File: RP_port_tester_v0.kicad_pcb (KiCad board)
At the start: 2 copper layers, 82 parts, among them J1 USB_B PORT0, J2 USB_B PORT1, J3 USB_B PORT2, J4 USB_B PORT3, J5 DE9_Pins, J6 DE9_Pins, J7 DE9_Pins, J8 DE9_Pins, J9 UART, Q1 IRLZ44N, SW1 BOOTSEL, U1 AMS1117-3.3, U2 STMPS2151, U3 STMPS2151, U4 FSUSB74MPX, U5 W25Q128JVS, U6 STMPS2151, U7 RP2040, U8 LM2904, Y1 ABM8-272-T3

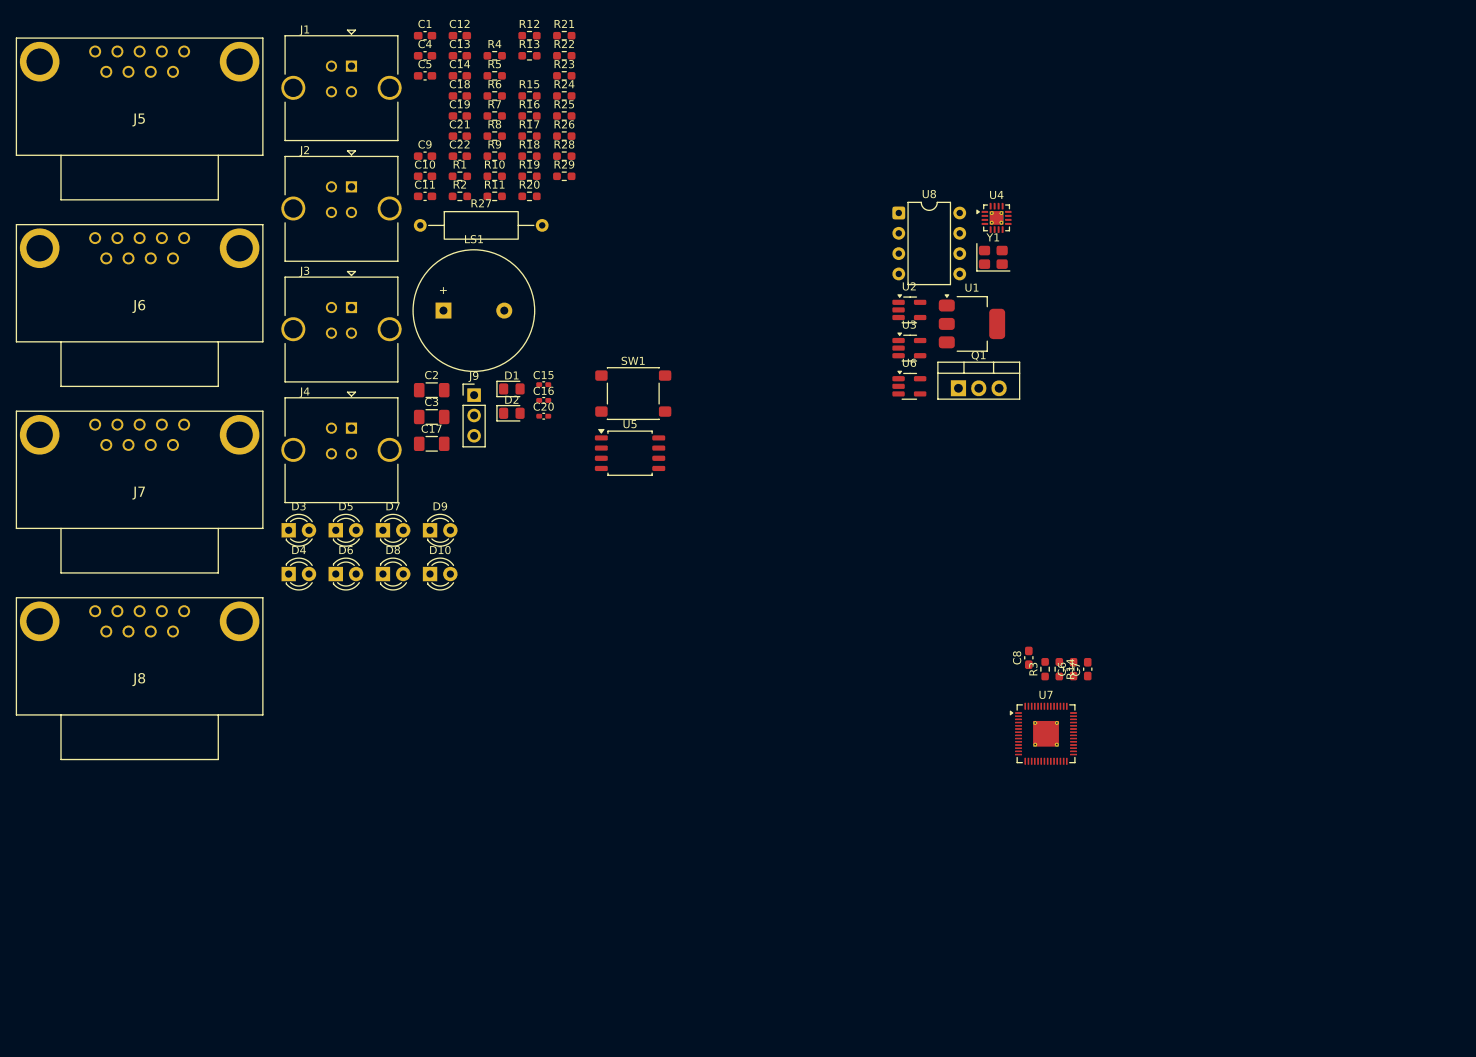
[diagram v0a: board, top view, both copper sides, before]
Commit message: Layout and Tracing
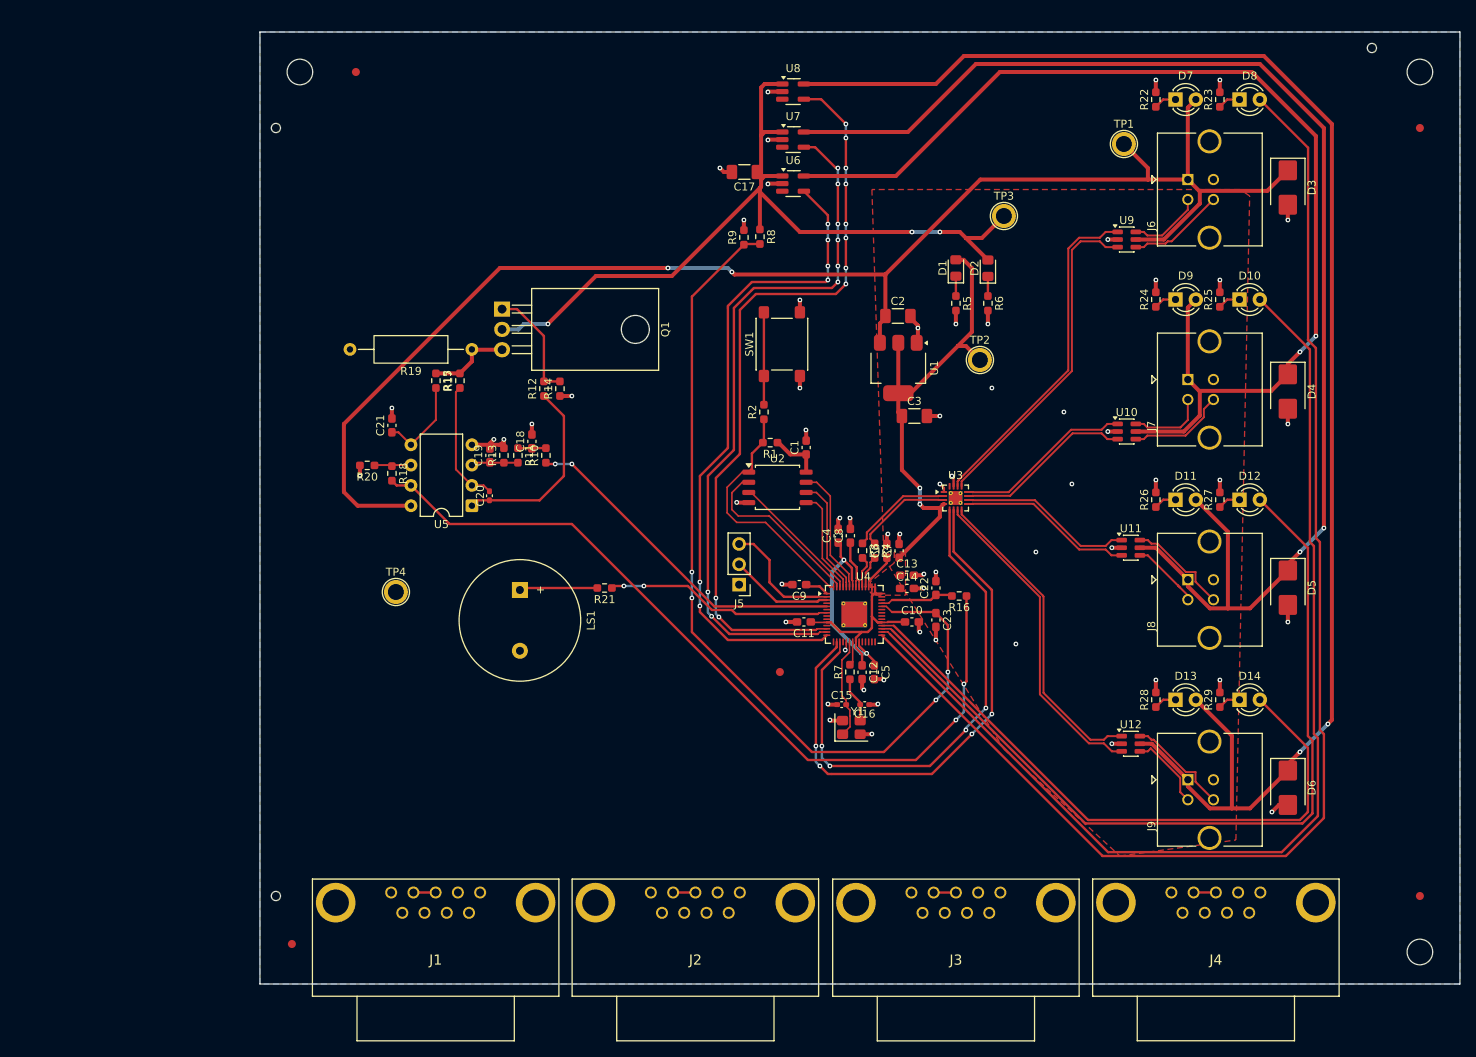
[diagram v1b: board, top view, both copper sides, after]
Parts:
- removed the J1 at (81.4, 29.3)
- removed the J2 at (81.4, 44.4)
- removed the J3 at (81.4, 59.4)
- removed the J4 at (81.4, 74.5)
- removed the R6 at (99.3, 33.0)
- removed the R7 at (99.3, 35.5)
- removed the U2 at (151.2, 59.7)
- removed the U3 at (151.2, 64.5)
- added C23: 100n, Capacitor_SMD:C_0603_1608Metric_Pad1.08x0.95mm_HandSolder, F.Cu at (154.5, 98.5)
- added D3: P6SMB6.8, Diode_SMD:D_SMB, F.Cu at (198.5, 44.4)
- added D4: P6SMB6.8, Diode_SMD:D_SMB, F.Cu at (198.5, 69.9)
- added D5: P6SMB6.8, Diode_SMD:D_SMB, F.Cu at (198.5, 94.5)
- added D6: P6SMB6.8, Diode_SMD:D_SMB, F.Cu at (198.5, 119.5)
- added FID1: Fiducial, Fiducial:Fiducial_1mm_Mask2mm, F.Cu at (74.0, 139.0)
- added FID2: Fiducial, Fiducial:Fiducial_1mm_Mask2mm, F.Cu at (82.0, 30.0)
- added FID3: Fiducial, Fiducial:Fiducial_1mm_Mask2mm, F.Cu at (215.0, 37.0)
- added FID4: Fiducial, Fiducial:Fiducial_1mm_Mask2mm, F.Cu at (215.0, 133.0)
- added FID5: Fiducial, Fiducial:Fiducial_1mm_Mask2mm, F.Cu at (135.0, 105.0)
- added H1: TOOLING_HOLE, MountingHole:ToolingHole_1.152mm, F.Cu at (209.0, 27.0)
- added H2: MountingHole, MountingHole:MountingHole_3.2mm_M3, F.Cu at (75.0, 30.0)
- added H3: TOOLING_HOLE, MountingHole:ToolingHole_1.152mm, F.Cu at (72.0, 37.0)
- added H4: MountingHole, MountingHole:MountingHole_3.2mm_M3, F.Cu at (215.0, 30.0)
- added H5: TOOLING_HOLE, MountingHole:ToolingHole_1.152mm, F.Cu at (72.0, 133.0)
- added H6: MountingHole, MountingHole:MountingHole_3.2mm_M3, F.Cu at (215.0, 140.0)
- added J6: USB_B PORT0, My_Library:USB_B_Vertical, F.Cu at (186.0, 43.4)
- added J7: USB_B PORT1, My_Library:USB_B_Vertical, F.Cu at (186.0, 68.4)
- added J8: USB_B PORT2, My_Library:USB_B_Vertical, F.Cu at (186.0, 93.5)
- added J9: USB_B PORT3, My_Library:USB_B_Vertical, F.Cu at (186.0, 118.5)
- added R14: 100k, Resistor_SMD:R_0603_1608Metric_Pad0.98x0.95mm_HandSolder, F.Cu at (107.5, 69.6)
- added R15: 1k, Resistor_SMD:R_0603_1608Metric_Pad0.98x0.95mm_HandSolder, F.Cu at (92.0, 68.6)
- added TP1: TestPoint, TestPoint:TestPoint_Plated_Hole_D2.0mm, F.Cu at (178.0, 39.0)
- added TP2: TestPoint, TestPoint:TestPoint_Plated_Hole_D2.0mm, F.Cu at (160.0, 66.0)
- added TP3: TestPoint, TestPoint:TestPoint_Plated_Hole_D2.0mm, F.Cu at (163.0, 48.0)
- added TP4: TestPoint, TestPoint:TestPoint_Plated_Hole_D2.0mm, F.Cu at (87.0, 95.0)
- added U10: USBLC6-2SC6, Package_TO_SOT_SMD:SOT-23-6, F.Cu at (178.4, 74.9)
- added U11: USBLC6-2SC6, Package_TO_SOT_SMD:SOT-23-6, F.Cu at (178.9, 89.5)
- added U12: USBLC6-2SC6, Package_TO_SOT_SMD:SOT-23-6, F.Cu at (178.9, 114.0)
- added U7: STMPS2151, Package_TO_SOT_SMD:SOT-23-5_HandSoldering, F.Cu at (136.7, 38.5)
- added U8: STMPS2151, Package_TO_SOT_SMD:SOT-23-5_HandSoldering, F.Cu at (136.7, 32.5)
- added U9: USBLC6-2SC6, Package_TO_SOT_SMD:SOT-23-6, F.Cu at (178.4, 50.9)
- Q1: footprint Package_TO_SOT_THT:TO-220-3_Vertical -> Package_TO_SOT_THT:TO-220-3_Horizontal_TabDown
- R10: value 220R -> 1k
- R11: value 390R -> 12k
- R12: value 220R -> 100R
- R13: value 390R -> 1k
- R16: value 70k -> 1k
- R17: value 100k -> 47R
- R18: value 1k -> 120k
- R19: value 12k -> 0R51; footprint Resistor_SMD:R_0603_1608Metric_Pad0.98x0.95mm_HandSolder -> Resistor_THT:R_Axial_DIN0309_L9.0mm_D3.2mm_P15.24mm_Horizontal
- R20: value 100R -> 10k
- R21: value 1k -> 100R
- R22: value 100k -> 220R
- R23: value 1k -> 390R
- R24: value 1k -> 220R
- R25: value 47R -> 390R
- R26: value 120k -> 220R
- R27: value 0R51 -> 390R; footprint Resistor_THT:R_Axial_DIN0309_L9.0mm_D3.2mm_P15.24mm_Horizontal -> Resistor_SMD:R_0603_1608Metric_Pad0.98x0.95mm_HandSolder
- R28: value 10k -> 220R
- R29: value 100R -> 390R
- R8: value 220R -> 70k
- R9: value 390R -> 100k
- moved J4 139.0 mm to (183.9, 132.6)
- moved D8 132.8 mm to (192.5, 33.4)
- moved D7 123.2 mm to (184.5, 33.4)
- moved D10 118.1 mm to (192.5, 58.4)
- moved J3 117.6 mm to (151.4, 132.6)
- moved J1 111.4 mm to (86.4, 132.6)
- moved D9 108.9 mm to (184.5, 58.4)
- moved D12 107.5 mm to (192.5, 83.5)
- moved J2 107.3 mm to (118.9, 132.6)
- moved R27 105.7 mm to (190.0, 83.5), turned to 90 degrees
- moved R29 104.9 mm to (190.0, 108.5), turned to 90 degrees
- moved D14 102.4 mm to (192.5, 108.5)
- moved R28 100.4 mm to (182.0, 108.5), turned to 90 degrees
- moved D11 99.2 mm to (184.5, 83.5)
- moved D13 95.6 mm to (184.5, 108.5)
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- renumbered D6 to D10, D7 to D11, D8 to D12, D9 to D13, D10 to D14, D3 to D7, D4 to D8, D5 to D9, J5 to J1, J6 to J2, J7 to J3, J8 to J4, J9 to J5, R14 to R4, R4 to R5, R5 to R6, R15 to R7, U5 to U2, U4 to U3, U7 to U4, U8 to U5
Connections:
- net /PICO_PORT0_TESTED renamed PICO_PORT0_TESTED
- net /PICO_PORT1_TESTED renamed PICO_PORT1_TESTED
- net /PICO_PORT2_TESTED renamed PICO_PORT2_TESTED
- net /PICO_PORT3_TESTED renamed PICO_PORT3_TESTED
- net /USB3_VBUS_EN renamed USB1_VBUS_EN
- net Net-(C16-Pad2) renamed /Crystal_Out
- net Net-(R2-Pad2) renamed /BOOTSEL_BTN
- net Net-(U7-XIN) renamed /PICO_XIN
- net Net-(U7-XOUT) renamed /PICO_XOUT
- C18 pad 1: Net-(C18-Pad1) -> /PWM_Filt
- C19 pad 1: Net-(U8A-+) -> /Amp Current+
- C20 pad 1: Net-(C20-Pad1) -> /Amp Current Out
- C20 pad 2: Net-(U8A--) -> /Amp Current-
- C21 pad 1: Net-(U8B-+) -> /Amp Gain+
- D10 pad 1: Net-(D6-K) -> Net-(D10-K)
- D11 pad 1: Net-(D7-K) -> Net-(D11-K)
- D11 pad 2: /USB2_VBUS -> /USB Connectors/USB2_VBUS
- D12 pad 1: Net-(D8-K) -> Net-(D12-K)
- D13 pad 1: Net-(D9-K) -> Net-(D13-K)
- D13 pad 2: /USB3_VBUS -> /USB Connectors/USB3_VBUS
- D14 pad 1: Net-(D10-K) -> Net-(D14-K)
- D7 pad 1: Net-(D3-K) -> Net-(D7-K)
- D8 pad 1: Net-(D4-K) -> Net-(D8-K)
- D9 pad 1: Net-(D5-K) -> Net-(D9-K)
- D9 pad 2: /USB1_VBUS -> /USB Connectors/USB1_VBUS
- Q1 pad 1: Net-(Q1-G) -> /FET-Gate
- Q1 pad 3: Net-(Q1-S) -> /Shunt High
- R10 pad 1: Net-(D7-K) -> /PICO_LOAD_PWM
- R10 pad 2: GND -> /PWM_Filt
- R11 pad 1: Net-(D8-K) -> /PWM_Filt
- R11 pad 2: GND -> /Amp Current+
- R12 pad 1: Net-(D9-K) -> /Amp Current Out
- R12 pad 2: GND -> /FET-Gate
- R13 pad 1: Net-(D10-K) -> /Amp Current+
- R16 pad 1: VBUS_TEST -> /Amp Gain Out
- R16 pad 2: /PICO_VBUS_ADC -> /PICO_CURRENT_ADC
- R17 pad 1: /PICO_VBUS_ADC -> /Amp Current-
- R17 pad 2: GND -> /Shunt High
- R18 pad 1: /PICO_LOAD_PWM -> /Amp Gain-
- R18 pad 2: Net-(C18-Pad1) -> /Amp Gain Out
- R19 pad 1: Net-(C18-Pad1) -> /Shunt High
- R19 pad 2: Net-(U8A-+) -> GND
- R20 pad 1: Net-(C20-Pad1) -> /Amp Gain-
- R20 pad 2: Net-(Q1-G) -> GND
- R21 pad 1: Net-(U8A-+) -> /PICO_AUDIO_EN
- R21 pad 2: GND -> Net-(LS1-Pad1)
- R22 pad 1: GND -> Net-(D7-K)
- R22 pad 2: Net-(Q1-G) -> GND
- R23 pad 1: Net-(Q1-S) -> Net-(D8-K)
- R23 pad 2: Net-(U8B-+) -> GND
- R24 pad 1: Net-(R24-Pad1) -> Net-(D9-K)
- R24 pad 2: /PICO_CURRENT_ADC -> GND
- R25 pad 1: Net-(U8A--) -> Net-(D10-K)
- R25 pad 2: Net-(Q1-S) -> GND
- R26 pad 1: Net-(U8B--) -> Net-(D11-K)
- R26 pad 2: Net-(R24-Pad1) -> GND
- R27 pad 1: Net-(Q1-S) -> Net-(D12-K)
- R28 pad 1: Net-(U8B--) -> Net-(D13-K)
- R29 pad 1: /PICO_AUDIO_EN -> Net-(D14-K)
- R29 pad 2: Net-(LS1-Pad1) -> GND
- R3 pad 1: /PICO_USB_D- -> /PICO_USB_D+
- R4 pad 1: /PICO_USB_D+ -> /PICO_USB_D-
- R8 pad 1: Net-(D5-K) -> VBUS_TEST
- R8 pad 2: GND -> /PICO_VBUS_ADC
- R9 pad 1: Net-(D6-K) -> /PICO_VBUS_ADC
- U3 pad 10: /USB2_D+ -> USB2_D+
- U3 pad 11: /USB1_D+ -> USB1_D+
- U3 pad 12: /USB1_D- -> USB1_D-
- U3 pad 13: /USB0_D+ -> USB0_D+
- U3 pad 14: /USB0_D- -> USB0_D-
- U3 pad 7: /USB3_D- -> USB3_D-
- U3 pad 8: /USB3_D+ -> USB3_D+
- U3 pad 9: /USB2_D- -> USB2_D-
- U4 pad 12: /USB1_VBUS_EN -> USB3_VBUS_EN
- U4 pad 13: /USB2_VBUS_EN -> USB2_VBUS_EN
- U4 pad 35: /PICO_AUDIO_EN -> unconnected-(U4-GPIO23-Pad35)
- U4 pad 5: unconnected-(U7-GPIO3-Pad5) -> /PICO_LOAD_PWM
- U4 pad 7: unconnected-(U7-GPIO5-Pad7) -> /PICO_AUDIO_EN
- U4 pad 8: /PICO_LOAD_PWM -> unconnected-(U4-GPIO6-Pad8)
- U5 pad 1: Net-(C20-Pad1) -> /Amp Current Out
- U5 pad 2: Net-(U8A--) -> /Amp Current-
- U5 pad 3: Net-(U8A-+) -> /Amp Current+
- U5 pad 5: Net-(U8B-+) -> /Amp Gain+
- U5 pad 6: Net-(U8B--) -> /Amp Gain-
- U5 pad 7: Net-(R24-Pad1) -> /Amp Gain Out
- U6 pad 5: /USB3_VBUS -> /USB Connectors/USB1_VBUS
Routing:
- net /USB Connectors/USB3_VBUS: track 0.00 -> 193.8 mm, vias 0 -> 2
- net VBUS: track 0.00 -> 186.9 mm, vias 0 -> 2
- net /USB Connectors/USB2_VBUS: track 0.00 -> 168.3 mm, vias 0 -> 2
- net PICO_PORT0_TESTED: track 0.00 -> 161.8 mm
- net /USB Connectors/USB1_VBUS: track 0.00 -> 140.2 mm, vias 0 -> 2
- net PICO_PORT1_TESTED: track 0.00 -> 135.3 mm
- net /PICO_VBUS_ADC: track 0.00 -> 111.8 mm, vias 0 -> 4
- net PICO_PORT2_TESTED: track 0.00 -> 106.4 mm
- net VBUS_TEST: track 0.00 -> 105.3 mm, vias 0 -> 3
- net /Amp Gain Out: track 0.00 -> 103.1 mm, vias 0 -> 2
- net +3.3V: track 0.00 -> 103.0 mm, vias 0 -> 2
- net USB3_VBUS_EN: track 0.00 -> 95.1 mm, vias 0 -> 10
- net USB2_VBUS_EN: track 0.00 -> 89.4 mm, vias 0 -> 8
- net GND: track 0.00 -> 88.5 mm, vias 0 -> 60
- net USB1_VBUS_EN: track 0.00 -> 83.4 mm, vias 0 -> 6
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- added copper zone on F.Cu, net +3.3V
- added copper zone on B.Cu, net GND
- added copper zone on F.Cu, net GND
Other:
- board outline added: 150 x 119 mm
